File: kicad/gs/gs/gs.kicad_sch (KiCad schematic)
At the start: 49 parts, among them J1 Jack_12V, J2 JST_MotorAz, J3 JST_MotorEl, J5 Breakout_DIP, J6 JST_ZeroAZ, U1 ESP32-WROOM-32-DEV, U2 MPU-9250-DEV, U3 Ai-Thinker-Ra-02, U4 L7805, U5 LD1117S33TR_SOT223, U6 L6219DS, U8 L6219DS, U9 ATGM332D-5N31-PCB

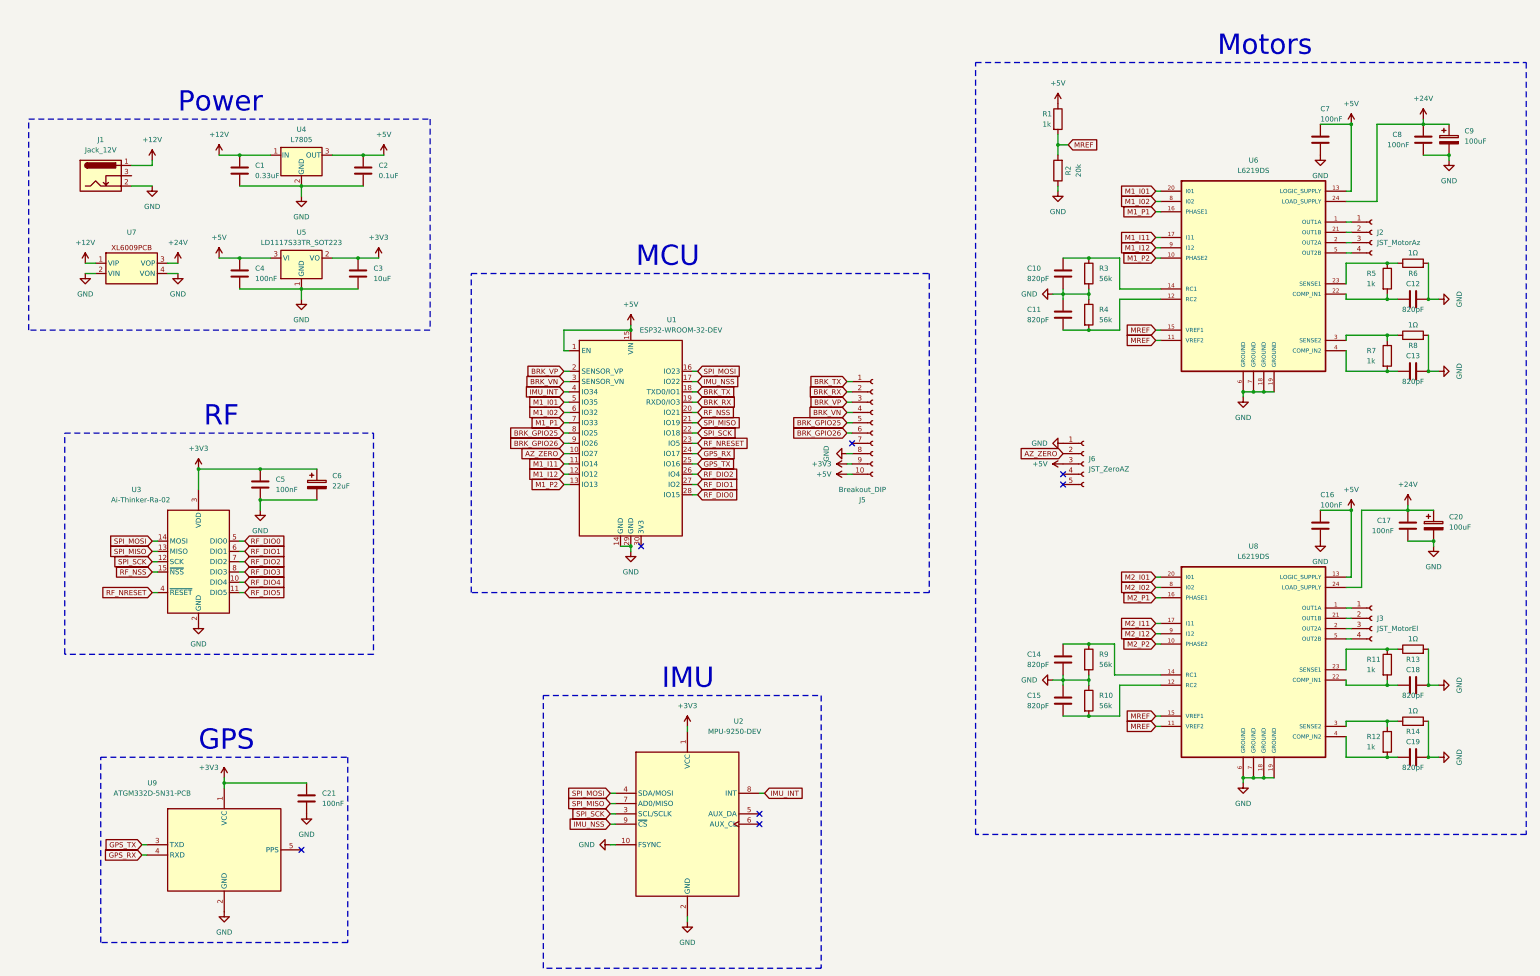
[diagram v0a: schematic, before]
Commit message: Finished second revision of GS PCB
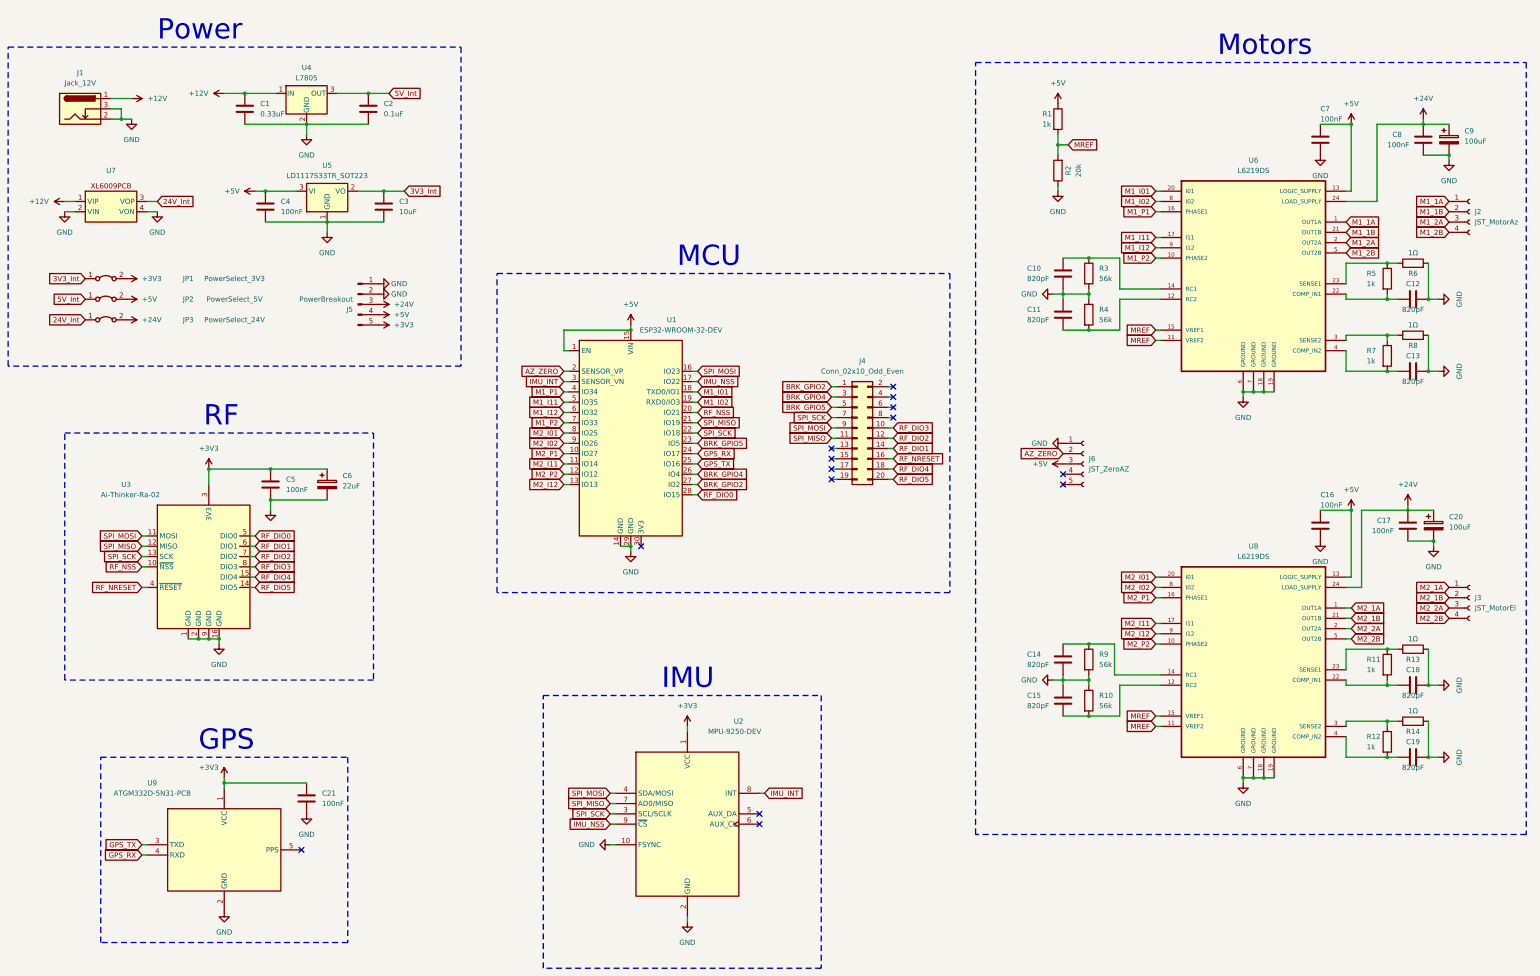
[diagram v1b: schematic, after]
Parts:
- removed J5: Breakout_DIP, Connector_PinSocket_2.54mm:PinSocket_1x10_P2.54mm_Vertical, symbol Connector:Conn_01x10_Socket
- added J4: Conn_02x10_Odd_Even, Connector_PinHeader_2.54mm:PinHeader_2x10_P2.54mm_Vertical, symbol Connector_Generic:Conn_02x10_Odd_Even
- added J5: PowerBreakout, Connector_PinHeader_2.54mm:PinHeader_1x05_P2.54mm_Vertical, symbol Connector:Conn_01x05_Pin
- added JP1: PowerSelect_3V3, Connector_PinHeader_2.54mm:PinHeader_1x02_P2.54mm_Vertical, symbol Jumper:Jumper_2_Bridged
- added JP2: PowerSelect_5V, Connector_PinHeader_2.54mm:PinHeader_1x02_P2.54mm_Vertical, symbol Jumper:Jumper_2_Bridged
- added JP3: PowerSelect_24V, Connector_PinHeader_2.54mm:PinHeader_1x02_P2.54mm_Vertical, symbol Jumper:Jumper_2_Bridged
- U3: footprint RF_Module:Ai-Thinker-Ra-01-LoRa -> RA-02-PCB:RA-02-PCB
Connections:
- net BRK_GPIO25 is gone; now on net M2_I01: U1.8 (IO25)
- net BRK_GPIO26 is gone; now on net M2_I02: U1.9 (IO26)
- net BRK_RX is gone; now on net M1_I02: U1.19 (RXD0/IO3)
- net BRK_TX is gone; now on net M1_I01: U1.18 (TXD0/IO1)
- net BRK_VN is gone; now on net IMU_INT: U1.3 (SENSOR_VN)
- net BRK_VP is gone; now on net AZ_ZERO: U1.2 (SENSOR_VP)
- net +24V: now also J5.3 (Pin_3), JP3.2 (B); no longer U7.3 (VOP)
- net +3V3: now also J5.5 (Pin_5), JP1.2 (B); no longer C3.1, U5.2 (VO)
- net +5V: now also J5.4 (Pin_4), JP2.2 (B); no longer C2.1, U4.3 (OUT)
- net AZ_ZERO: no longer U1.10 (IO27)
- net GND: now also J1.3, J5.1 (Pin_1), J5.2 (Pin_2)
- net IMU_INT: no longer U1.4 (IO34)
- net M1_I01: no longer U1.5 (IO35)
- net M1_I02: no longer U1.6 (IO32)
- net M1_I11: now also U1.5 (IO35); no longer U1.11 (IO14)
- net M1_I12: now also U1.6 (IO32); no longer U1.12 (IO12)
- net M1_P1: now also U1.4 (IO34); no longer U1.7 (IO33)
- net M1_P2: now also U1.7 (IO33); no longer U1.13 (IO13)
- net M2_I11: now also U1.11 (IO14)
- net M2_I12: now also U1.13 (IO13)
- net M2_P1: now also U1.10 (IO27)
- net M2_P2: now also U1.12 (IO12)
- net RF_DIO1: now also J4.14 (Pin_14); no longer U1.27 (IO2)
- net RF_DIO2: now also J4.12 (Pin_12); no longer U1.26 (IO4)
- net RF_DIO3: now also J4.10 (Pin_10)
- net RF_DIO4: now also U3.15 (DIO4), J4.18 (Pin_18); no longer U3.10 (DIO4)
- net RF_DIO5: now also U3.14 (DIO5), J4.20 (Pin_20); no longer U3.11 (DIO5)
- net RF_NRESET: now also J4.16 (Pin_16); no longer U1.23 (IO5)
- net RF_NSS: now also U3.10 (~{NSS}); no longer U3.15 (~{NSS})
- net SPI_MISO: now also U3.12 (MISO), J4.11 (Pin_11); no longer U3.13 (MISO)
- net SPI_MOSI: now also U3.11 (MOSI), J4.9 (Pin_9); no longer U3.14 (MOSI)
- net SPI_SCK: now also U3.13 (SCK), J4.7 (Pin_7); no longer U3.12 (SCK)
- net M2_1A: now reaches J3.1 (Pin_1), U8.1 (OUT1A)
- net M2_1B: now reaches J3.2 (Pin_2), U8.21 (OUT1B)
- net M2_2A: now reaches J3.3 (Pin_3), U8.2 (OUT2A)
- net M2_2B: now reaches J3.4 (Pin_4), U8.5 (OUT2B)
- net M1_1A: now reaches J2.1 (Pin_1), U6.1 (OUT1A)
- net M1_2A: now reaches J2.3 (Pin_3), U6.2 (OUT2A)
- net M1_1B: now reaches J2.2 (Pin_2), U6.21 (OUT1B)
- net M1_2B: now reaches J2.4 (Pin_4), U6.5 (OUT2B)
- new net 24V_Int: JP3.1 (A), U7.3 (VOP)
- new net 3V3_Int: C3.1, JP1.1 (A), U5.2 (VO)
- new net 5V_Int: C2.1, JP2.1 (A), U4.3 (OUT)
- new net BRK_GPIO2: J4.1 (Pin_1), U1.27 (IO2)
- new net BRK_GPIO4: J4.3 (Pin_3), U1.26 (IO4)
- new net BRK_GPIO5: J4.5 (Pin_5), U1.23 (IO5)
- no-connect marks 7 -> 14
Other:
- moved on the sheet: C1, C2, C3, C4, C5, C6, J1, J2, U4, U5, U7
